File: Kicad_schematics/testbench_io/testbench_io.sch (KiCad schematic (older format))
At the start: 43 parts, among them J101 Conn_01x02, J102 Conn_01x02, J103 Conn_01x02, J104 DB37_Female_MountingHoles, SW101 SW_SPST, SW102 SW_Push, SW103 SW_Push, SW104 SW_Push, SW105 SW_Push, SW106 SW_SPST, SW107 SW_SPST, SW108 SW_DIP_x08, SW109 SW_SPST, SW110 SW_Push, SW111 SW_SPST, SW112 SW_SPST, SW113 SW_SPST, SW114 SW_DPDT_x2, U101 NUCLEO64-F476RG, U102 CJMCU_MCP2551

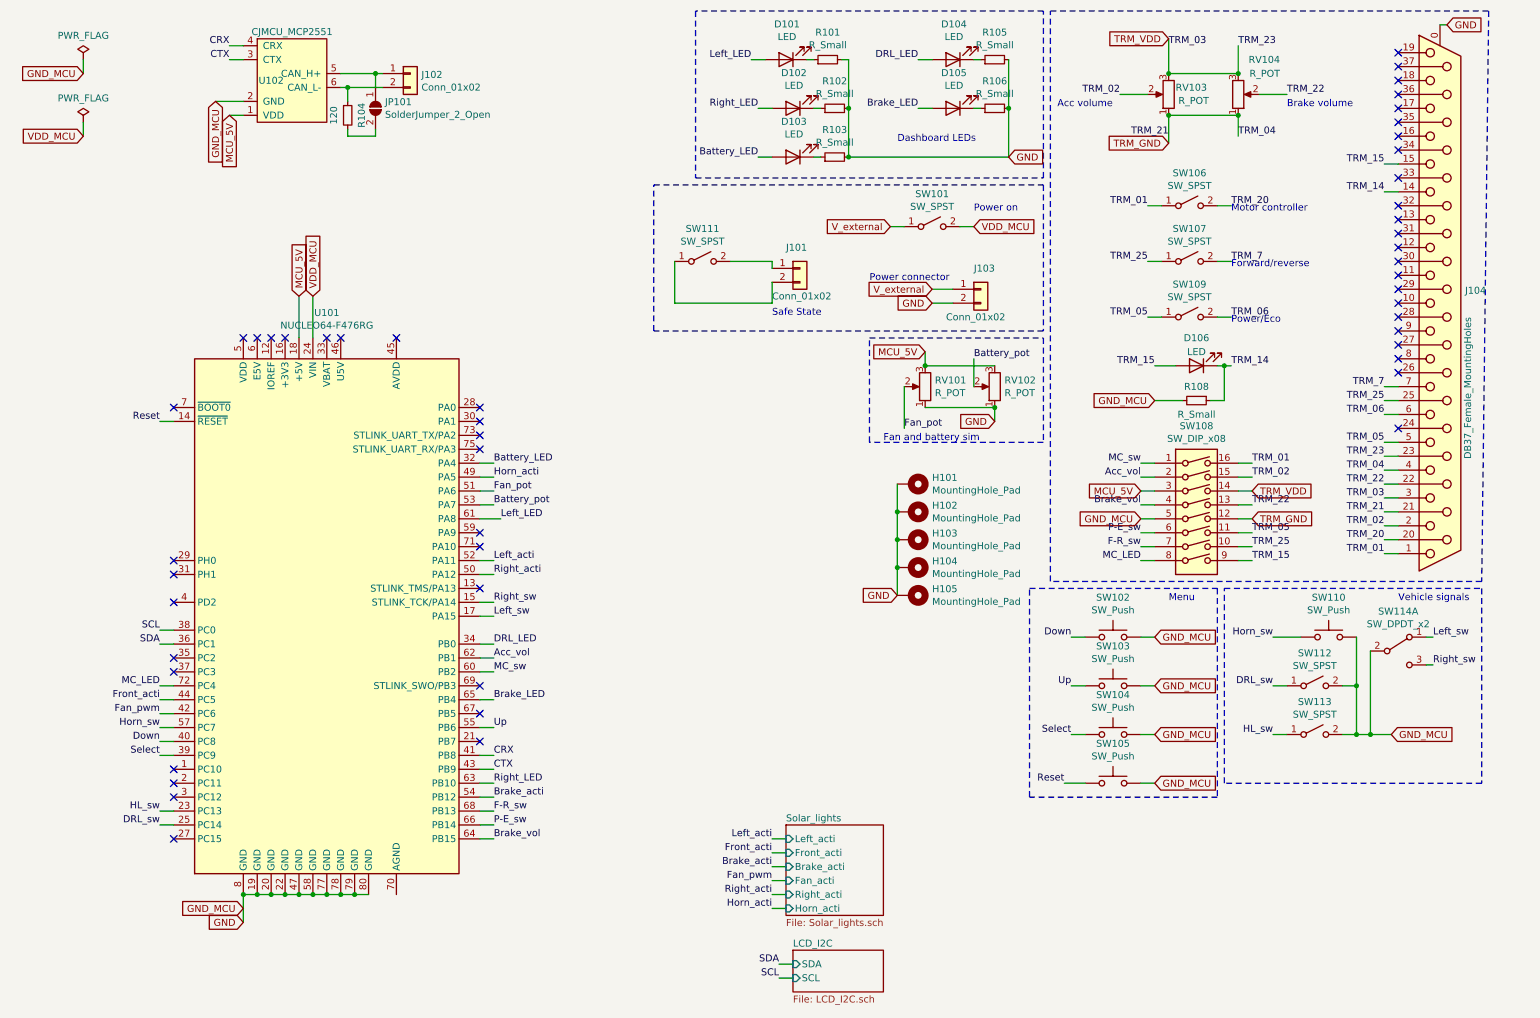
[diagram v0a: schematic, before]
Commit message: Fixed gerbers
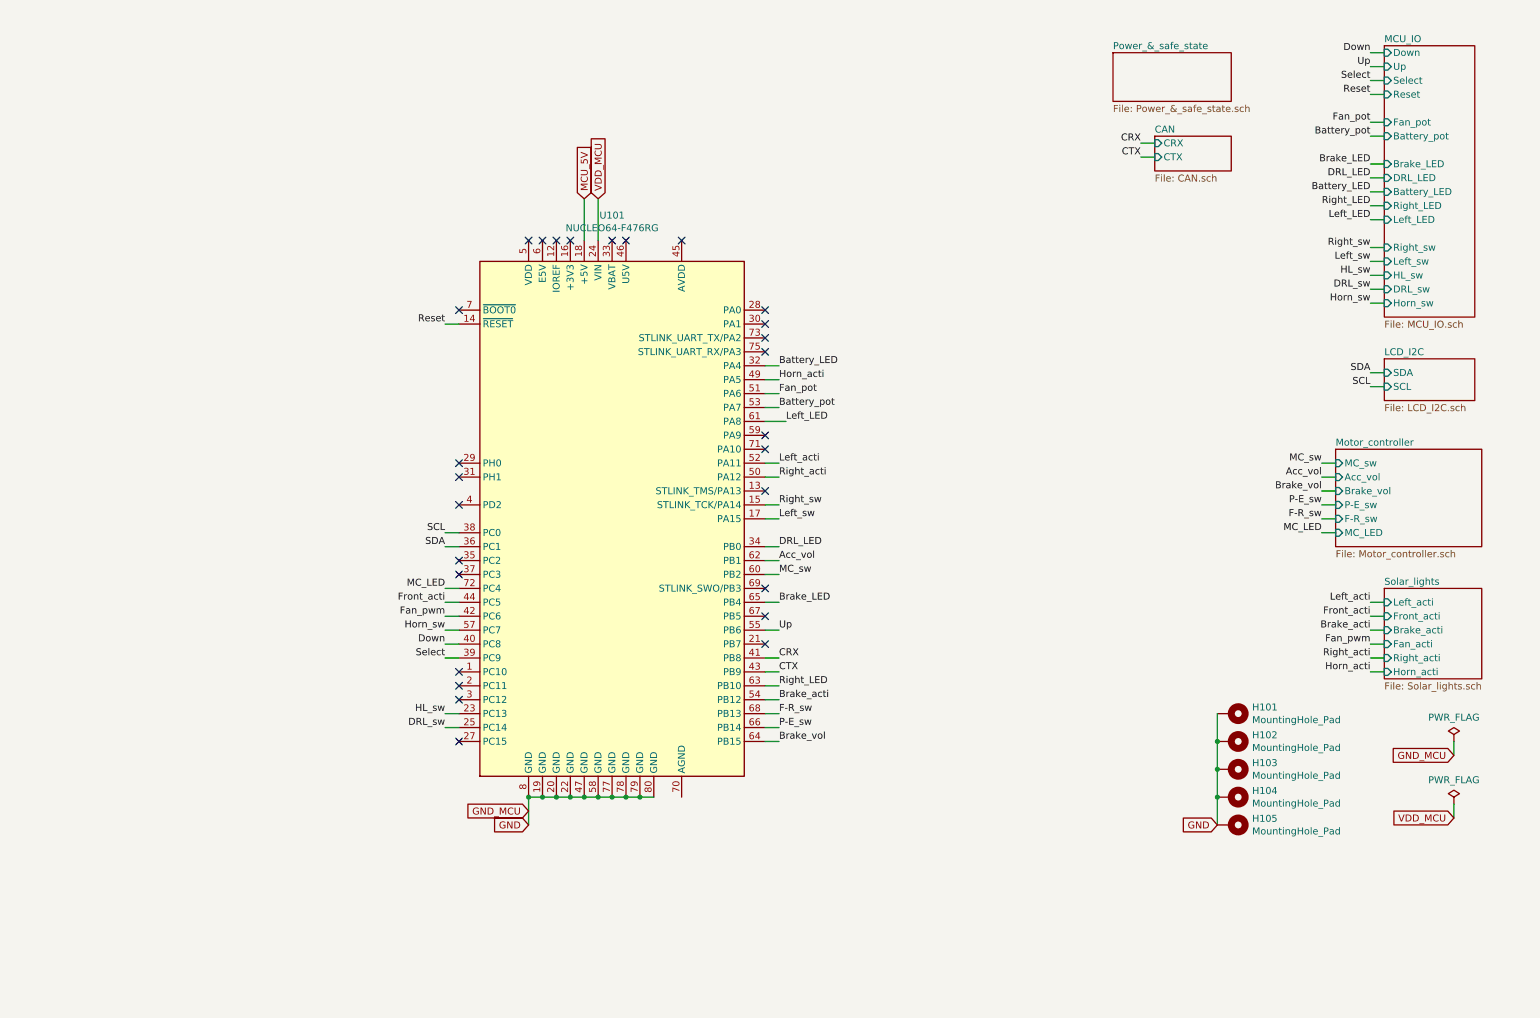
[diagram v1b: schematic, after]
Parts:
- removed D101, D102, D103, D104, D105, D106: LED, LED_THT:LED_D5.0mm, symbol Device:LED
- removed J101, J102, J103: Conn_01x02, Connector_JST:JST_XH_S2B-XH-A_1x02_P2.50mm_Horizontal, symbol Connector_Generic:Conn_01x02
- removed J104: DB37_Female_MountingHoles, Connector_Dsub:DSUB-37_Female_Horizontal_P2.77x2.84mm_EdgePinOffset7.70mm_Housed_MountingHolesOffset9.12mm, symbol Connector:DB37_Female_MountingHoles
- removed JP101: SolderJumper_2_Open, Jumper:SolderJumper-2_P1.3mm_Open_Pad1.0x1.5mm, symbol Jumper:SolderJumper_2_Open
- removed R101, R102, R103, R105, R106, R108: R_Small, Resistor_SMD:R_0603_1608Metric, symbol Device:R_Small
- removed R104: 120, Resistor_SMD:R_0603_1608Metric, symbol Device:R_Small
- removed RV101, RV102, RV103, RV104: R_POT, Potentiometer_THT:Potentiometer_Bourns_PTV09A-1_Single_Vertical, symbol Device:R_POT
- removed SW101, SW106, SW107, SW109, SW111, SW112, SW113: SW_SPST, Solar_team:RND-Slide-Switch, symbol Switch:SW_SPST
- removed SW102, SW103, SW104, SW105, SW110: SW_Push, Button_Switch_THT:SW_PUSH-12mm, symbol Switch:SW_Push
- removed SW108: SW_DIP_x08, Package_DIP:DIP-16_W7.62mm, symbol Switch:SW_DIP_x08
- removed SW114: SW_DPDT_x2, Solar_team:RND-Slide-Switch, symbol Switch:SW_DPDT_x2
- removed U102: CJMCU_MCP2551, Solar_team:CJMCU_2551, symbol Solarteam:CJMCU_MCP2551
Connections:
- no-connect marks 50 -> 27
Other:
- note removed: "Acc volume\n"
- note removed: "Brake volume\n"
- note removed: "Dashboard LEDs\n"
- note removed: "Fan and battery sim"
- note removed: "Forward/reverse\n"
- note removed: "Menu"
- note removed: "Motor controller\n"
- note removed: "Power connector\n"
- note removed: "Power on\n"
- note removed: "Power/Eco\n"
- note removed: "Safe State\n"
- note removed: "Vehicle signals"
- moved on the sheet: H101, H102, H103, H104, H105, U101
